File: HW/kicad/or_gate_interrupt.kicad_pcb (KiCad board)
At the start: 2 copper layers, 24.4 x 45.2 mm, 12 parts, among them P1 G_G_G_I1_I2_V, P2 GND_GP0, P3 Rx_Tx, U1 74LS32, U2 74HC02, U3 ESP-01v090, U4 LT1129CST-3.3

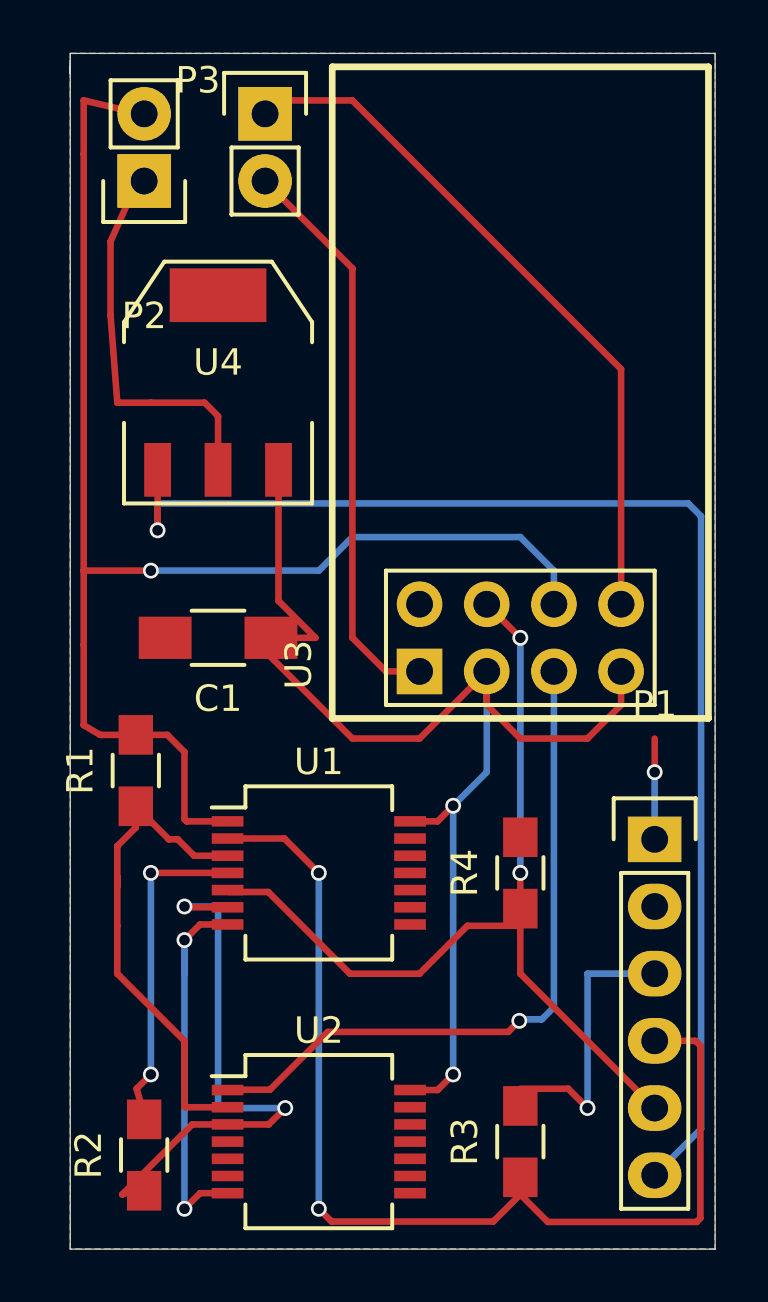
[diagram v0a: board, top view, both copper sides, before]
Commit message: Sending this to the FAB, after opening and checking.
V1
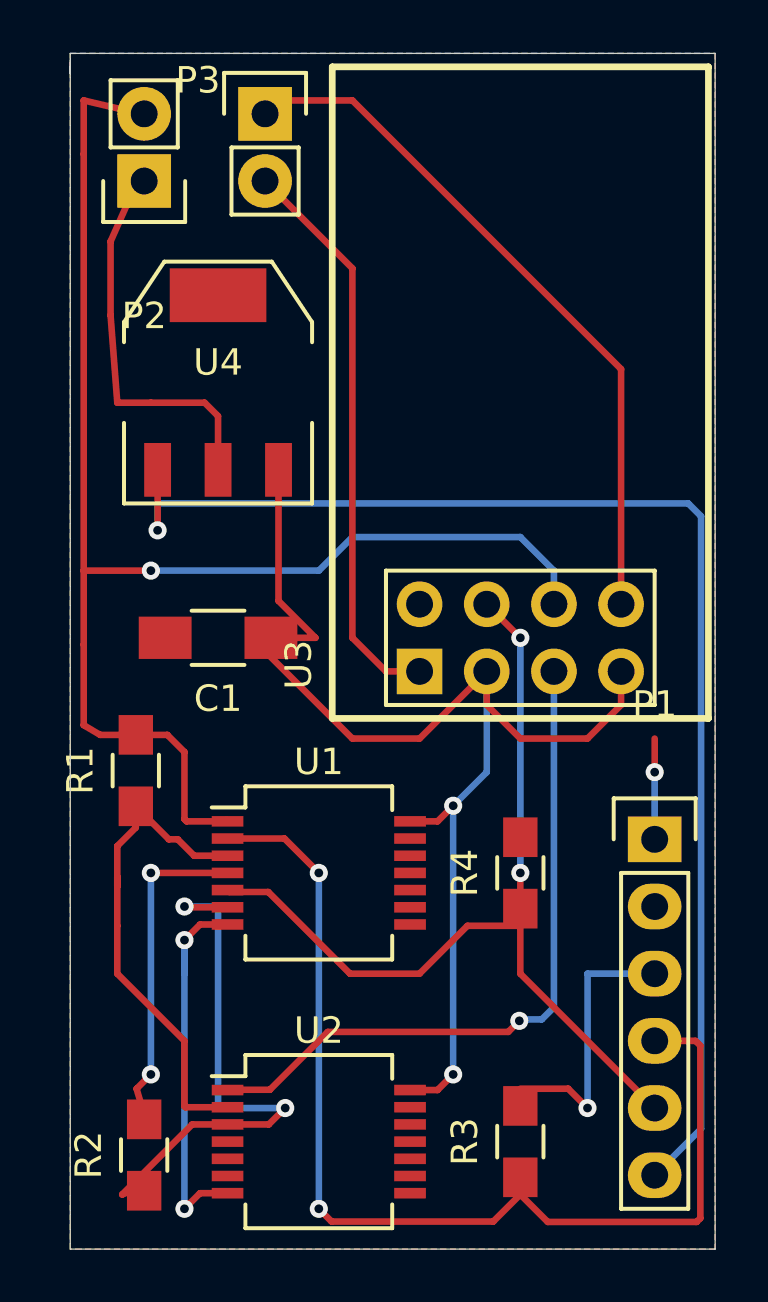
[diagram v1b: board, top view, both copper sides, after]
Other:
- net class Default: via_dia 0.6 -> 0.6858; via_drill 0.4 -> 0.3302
- rule via_min_drill: 0.3 -> 0.3302
- rule via_min_size: 0.4 -> 0.6858
